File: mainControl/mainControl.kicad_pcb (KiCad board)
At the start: 4 copper layers, 50 x 50 mm, 128 parts, among them J1 USB_B_Micro, J10 USB_B_Micro, J11 Conn_01x02, J12 Conn_01x02, J2 Conn_01x03, J3 Conn_01x02, J4 Conn_01x02, J5 Conn_01x03, J6 Conn_01x03, J7 Conn_01x03, J8 Conn_01x03, J9 Conn_01x04, Q1 MMBT3904LP, Q2 MMBT3904LP, U1 W25Q16JVUXIQ, U10 MCP3465R, U2 RP2040, U3 INA186A3IDDF, U4 ILPS22QS, U5 AP63357Q, U6 MCP79410T-I/MNY, U7 ESP32-WROOM-32, U8 CP2102N-Axx-xQFN24, U9 TVS2700DRV, Y1 12Mhz, Y2 Crystal

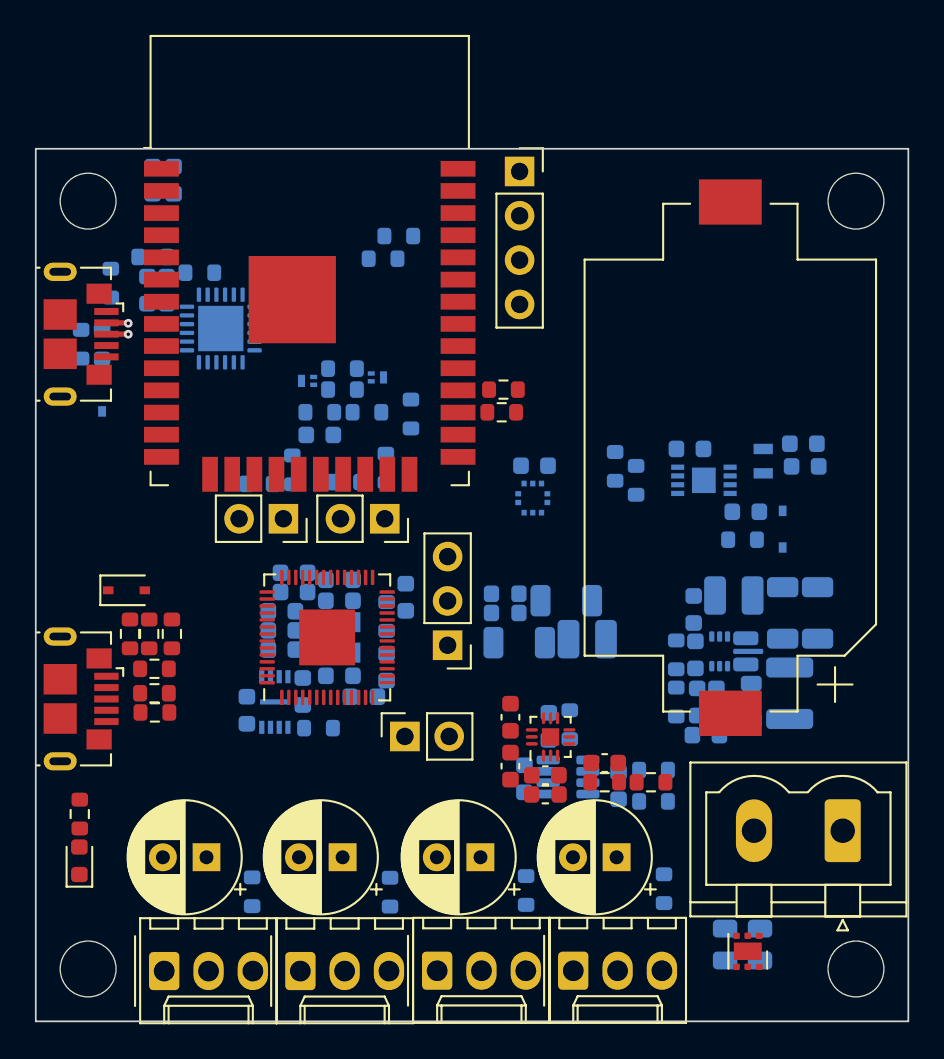
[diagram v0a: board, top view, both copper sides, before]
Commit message: wip
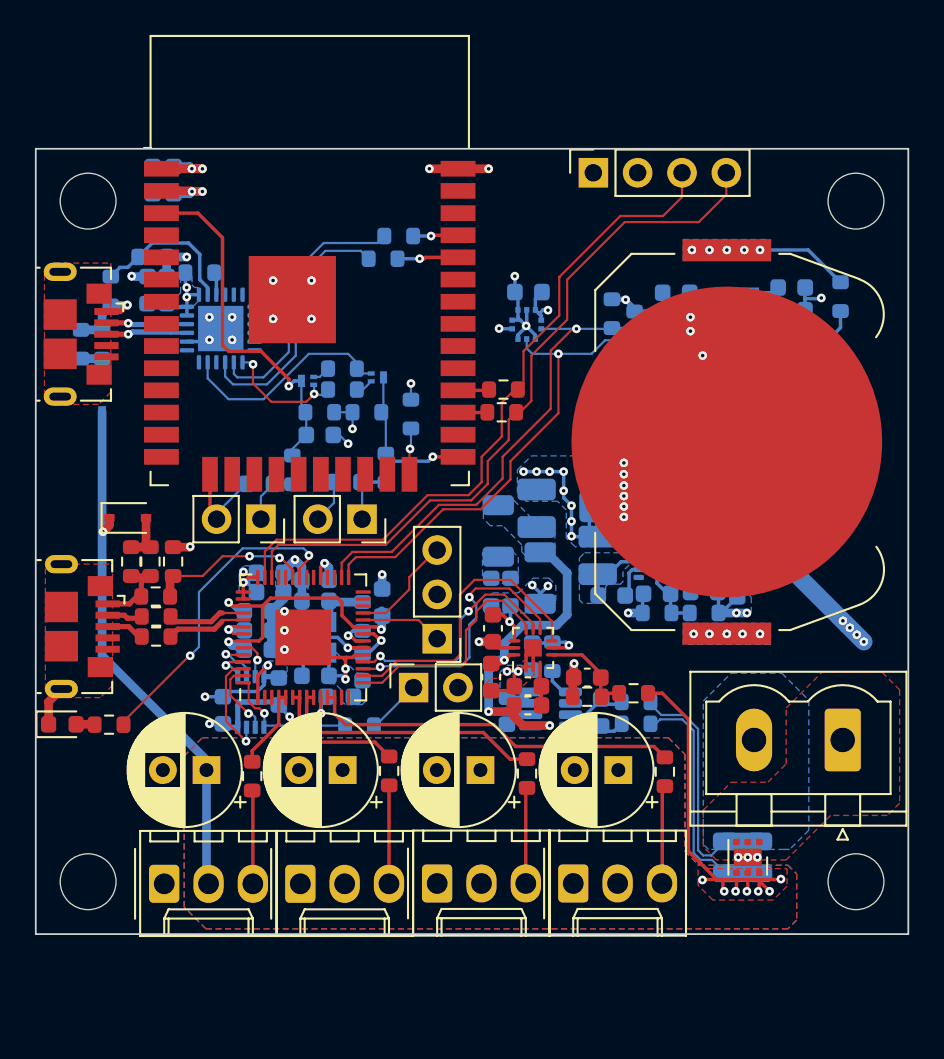
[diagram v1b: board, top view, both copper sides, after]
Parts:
- BT1: footprint Battery:BatteryHolder_Keystone_1060_1x2032 -> Battery:BatteryHolder_Keystone_3034_1x20mm
- R16, R17, R18, R19: moved to F.Cu
- moved R26 15.0 mm to (116.1, 140.5), turned to -90 degrees
- moved C33 14.1 mm to (103.2, 150.5), turned to 180 degrees
- moved C13 12.5 mm to (107.5, 152.1), turned to 0 degrees
- moved C31 11.4 mm to (103.2, 152.5), turned to 180 degrees
- moved D3 10.1 mm to (113.0, 143.8), turned to 0 degrees
- moved C14 9.96 mm to (98.2, 140.2)
- moved U4 9.96 mm to (98.2, 142.1)
- moved L1 9.75 mm to (108.4, 154.3), turned to 0 degrees
- moved C30 8.98 mm to (109.9, 143.8)
- moved Y2 8.98 mm to (110.9, 140.9)
- moved C12 8.98 mm to (106.7, 140.2)
- moved C26 8.98 mm to (113.3, 141.2)
- moved U6 8.98 mm to (107.5, 142.1)
- moved C28 8.98 mm to (113.3, 139.9)
- moved C19 8.88 mm to (110.2, 156.9), turned to 90 degrees
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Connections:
- J9 pad 3: /termUART_RX -> /ESP/RXD
- J9 pad 4: /termUART_TX -> /ESP/TXD
- U2 pad 11: /UART3 -> /UART0
- U2 pad 12: /UART3 -> /UART0
- U2 pad 4: /UART0 -> /UART3
- U2 pad 5: /UART0 -> /UART3
- U2 pad 6: /UART1 -> /UART2
- U2 pad 7: /UART1 -> /UART2
- U2 pad 8: /UART2 -> /UART1
- U2 pad 9: /UART2 -> /UART1
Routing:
- net GND: track 0.00 -> 112.1 mm, vias 0 -> 48
- net +24V: track 0.00 -> 99.7 mm, vias 0 -> 12
- net +3V3: track 0.00 -> 58.0 mm, vias 0 -> 27
- net Net-(BT1-Pad1): track 0.00 -> 43.1 mm, vias 0 -> 10
- net /ESP/TXD: track 0.00 -> 41.6 mm
- net /ESP/RXD: track 0.00 -> 39.6 mm
- net /pheri/SCL: track 0.00 -> 29.6 mm, vias 0 -> 1
- net /pheri/SDA: track 0.00 -> 29.3 mm, vias 0 -> 1
- net /UART0: track 0.00 -> 21.3 mm
- net /ESP/ESP_EN: track 0.00 -> 20.8 mm, vias 0 -> 1
- net +3.3VA: track 0.00 -> 20.2 mm, vias 0 -> 3
- net Net-(R10-Pad1): track 0.00 -> 18.5 mm, vias 0 -> 2
- net +1V1: track 0.00 -> 17.3 mm, vias 0 -> 3
- net /pheri/CS: track 0.00 -> 17.2 mm
- net /pheri/SCK: track 0.00 -> 15.8 mm, vias 0 -> 2
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- added copper zone on B.Cu, net +24V
- added copper zone on F.Cu, net +24V
- added copper zone on B.Cu, net +3.3VA
- added copper zone on B.Cu, net +3V3
- added copper zone on In2.Cu, net +3V3
- added copper zone on B.Cu, net GND
- added copper zone on F.Cu, net GND
- added copper zone on In1.Cu, net GND
- added copper zone on In2.Cu, net GND
- added copper zone on B.Cu, net Net-(BT1-Pad1)
- added copper zone on B.Cu, net Net-(C13-Pad2)
- added copper zone on B.Cu, net Net-(C20-Pad1)
- added copper zone on B.Cu, net Net-(C45-Pad1)
- added copper zone on B.Cu, net Net-(J4-Pad2)
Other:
- board size 50 x 50 mm -> 50 x 45 mm
